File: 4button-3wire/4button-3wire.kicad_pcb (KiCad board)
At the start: 2 copper layers, 72 x 25.5 mm, 10 parts, among them J1 PCB Audio Jack, SW1 SW_Push_LED_Separate, SW2 SW_Push_LED_Separate, SW3 SW_Push_LED_Separate, SW4 SW_Push_LED_Separate

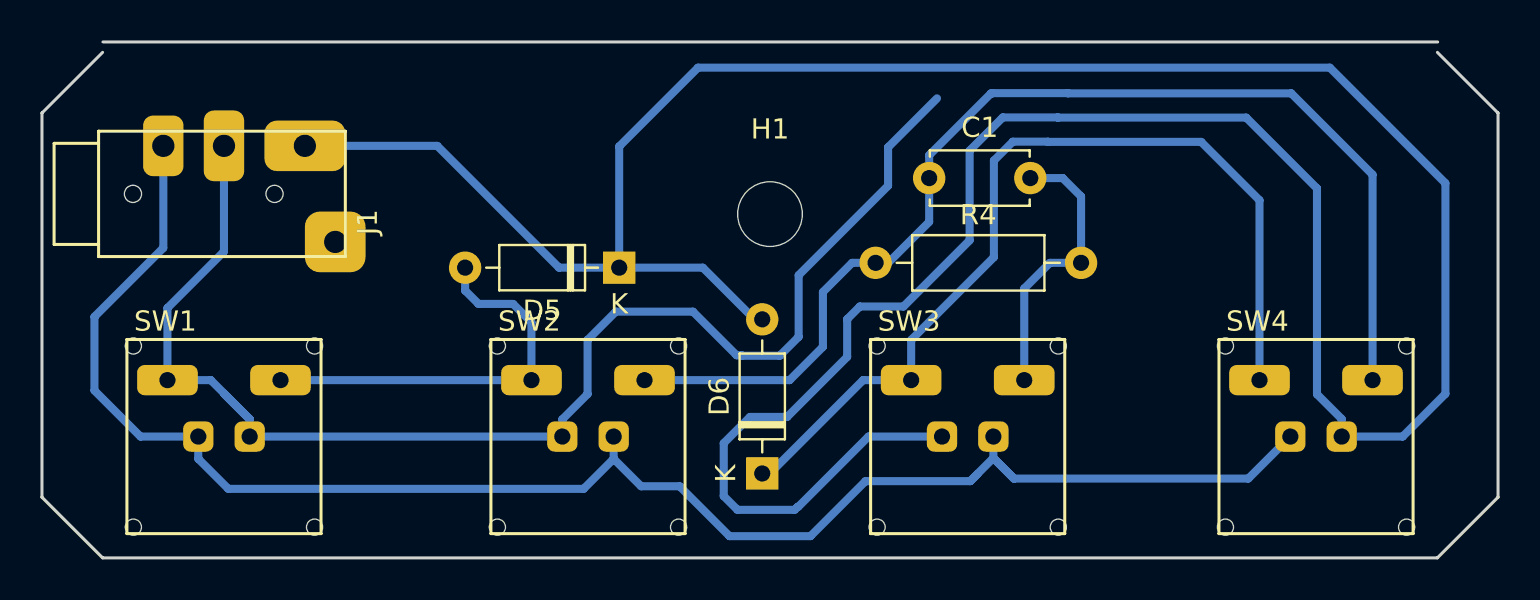
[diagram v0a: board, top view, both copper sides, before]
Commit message: First milled PCB revision
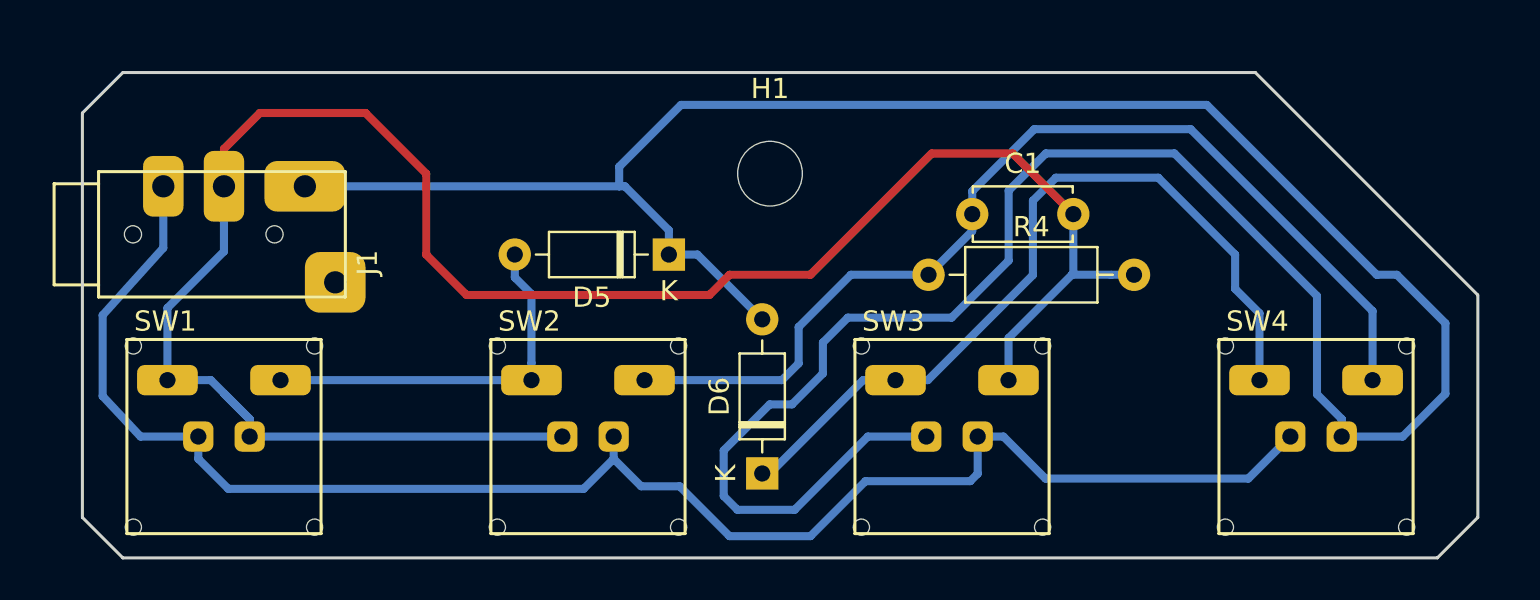
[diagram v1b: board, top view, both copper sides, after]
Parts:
- moved C1 2.78 mm to (113.0, 103.0)
- moved R4 2.68 mm to (110.8, 106.0)
- moved D5 2.54 mm to (98.0, 105.0)
- moved H1 2.00 mm to (103.0, 101.0)
- moved J1 2.00 mm to (82.0, 104.0)
- moved SW3 0.78 mm to (112.0, 114.0)
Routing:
- net Net-(C1-Pad2): track 82.0 -> 101.1 mm
- net Net-(D5-Pad1): track 163.5 -> 145.9 mm
- net Net-(C1-Pad1): track 57.2 -> 50.5 mm
- net Net-(D6-Pad1): track 44.9 -> 40.1 mm
- net Net-(J1-PadS): track 84.4 -> 81.0 mm
- net Net-(D5-Pad2): track 20.3 -> 19.0 mm
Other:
- board size 72 x 25.5 mm -> 69 x 24 mm
